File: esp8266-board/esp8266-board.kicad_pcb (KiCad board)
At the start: 2 copper layers, 58.7 x 58.7 mm, 20 parts, among them J1 PGM, J2 StepDown-3A, J3 LED, J4 USB, J5 Barrel_Jack, U1 ESP-12E

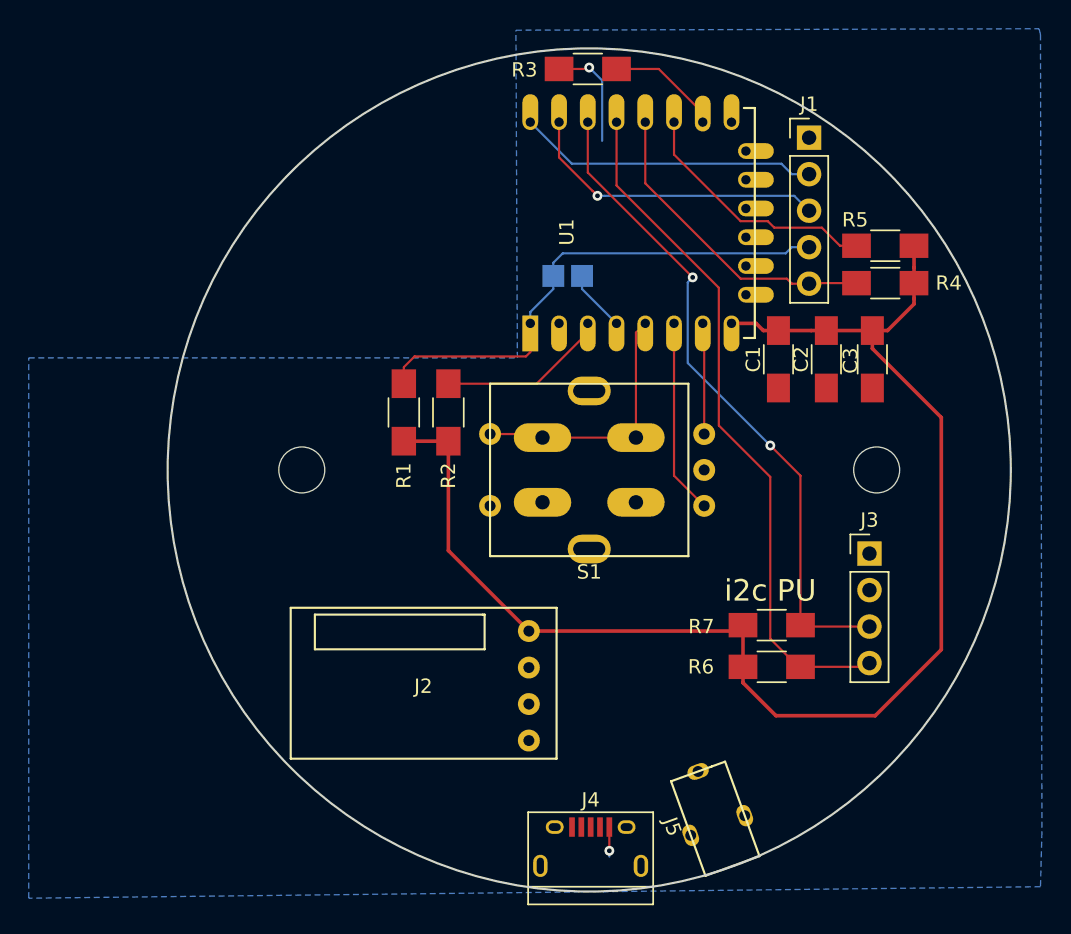
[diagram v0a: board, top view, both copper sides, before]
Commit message: First board rev order 0.1
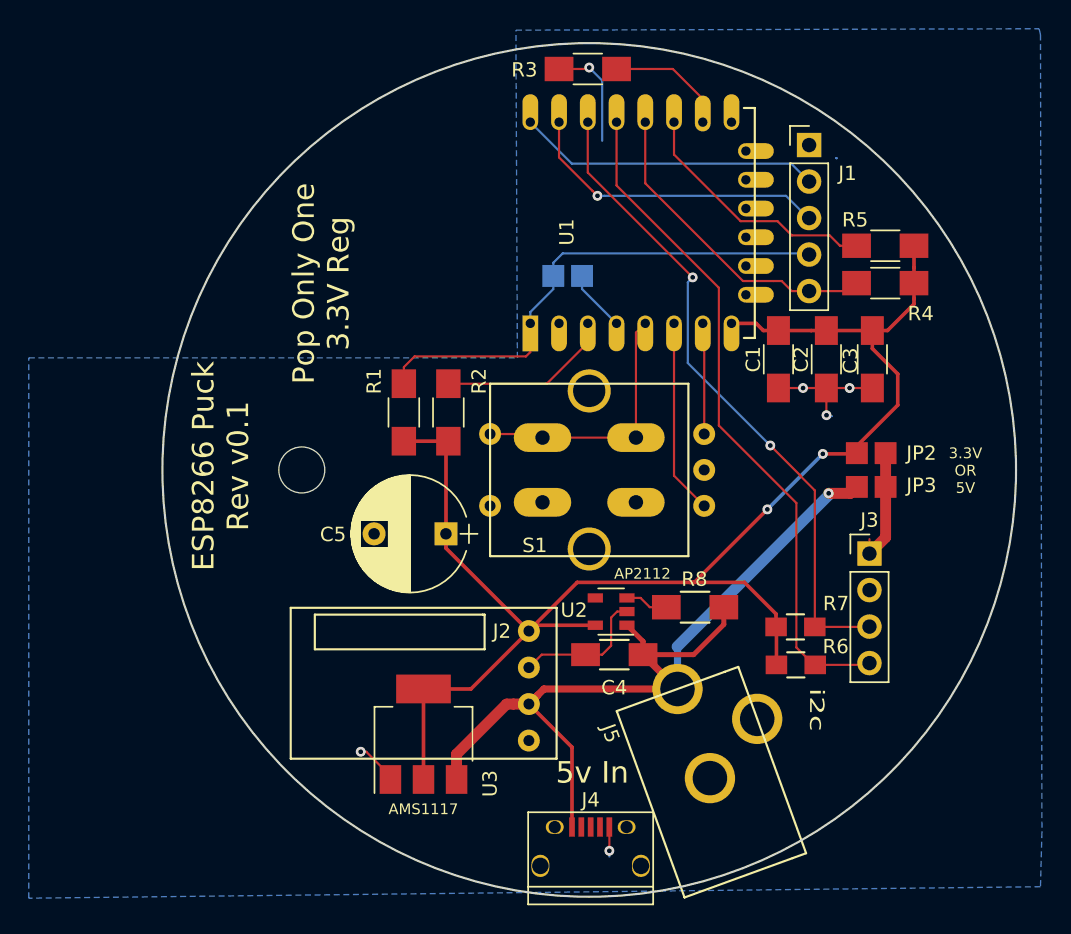
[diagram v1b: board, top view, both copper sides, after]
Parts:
- removed the REF** at (164.0, 102.0)
- added C4: 10uF, Capacitors_SMD:C_1206_HandSoldering, F.Cu at (145.7, 114.9)
- added C5: 300uF, Capacitors_THT:CP_Radial_D8.0mm_P5.00mm, F.Cu at (134.0, 106.4)
- added JP2: 3.3V, Features:SolderJumper, F.Cu at (163.6, 100.8)
- added JP3: 5V, Features:SolderJumper, F.Cu at (163.6, 103.2)
- added R8: 10k, Resistors_SMD:R_1206_HandSoldering, F.Cu at (151.4, 111.6)
- added U2: AP2112, TO_SOT_Packages_SMD:SOT-23-5, F.Cu at (145.5, 111.9)
- added U3: AMS1117-3.3, TO_SOT_Packages_SMD:SOT-223, F.Cu at (132.5, 120.4)
- J4: footprint Connectors:USB_Micro-B -> Power:USB_Micro-B
- R6, R7: footprint Resistors_SMD:R_1206_HandSoldering -> Resistors_SMD:R_0805_HandSoldering
- moved R6 1.68 mm to (158.4, 115.6)
- moved R7 1.65 mm to (158.3, 112.9)
- moved J5 1.16 mm to (152.8, 124.7)
- moved J1 0.51 mm to (159.3, 79.4)
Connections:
- J2 pad 1: Net-(J2-Pad1) -> (no net)
- J3 pad 1: +5V -> Net-(J3-Pad1)
- J4 pad 2: Net-(J4-Pad2) -> (no net)
- J4 pad 3: Net-(J4-Pad3) -> (no net)
- J4 pad 4: Net-(J4-Pad4) -> (no net)
- J5 pad 3: Net-(J5-Pad3) -> GND
- U1 pad 17: Net-(U1-Pad17) -> (no net)
- U1 pad 18: Net-(U1-Pad18) -> (no net)
- U1 pad 19: Net-(U1-Pad19) -> (no net)
- U1 pad 2: ADC -> (no net)
- U1 pad 20: Net-(U1-Pad20) -> (no net)
- U1 pad 21: Net-(U1-Pad21) -> (no net)
- U1 pad 22: Net-(U1-Pad22) -> (no net)
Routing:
- net +5V: track 0.00 -> 64.8 mm, vias 0 -> 1
- net GND: track 9.66 -> 31.1 mm, vias 2 -> 6
- net Net-(J3-Pad1): track 0.00 -> 9.37 mm
- net +3V3: track 96.3 -> 105.4 mm, vias 0 -> 2
- net Net-(R8-Pad2): track 0.00 -> 3.92 mm
- net Net-(R3-Pad2): track 7.91 -> 8.48 mm
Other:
- board size 58.7 x 58.7 mm -> 59.4 x 59.4 mm
- net class 5V PWR: clearance 0.762 -> 0.254; trace_width 0.762 -> 0.5
- board text added: "3.3V OR 5V"
- board text added: "5v In"
- board text added: "AMS1117"
- board text added: "AP2112"
- board text added: "ESP8266 Puck Rev v0.1"
- board text added: "Pop Only One 3.3V Reg"
- board text added: "i2c"
- board text removed: "i2c PU"
